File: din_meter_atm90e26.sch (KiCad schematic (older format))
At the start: 45 parts, among them J1 PCIx1, J2 Conn_01x05, J5 CONN_01X10, M1 ATM90E26_ATM90E26, M2 ATM90E26_ATM90E26, Y1 Crystal_Small, Y2 Crystal_Small

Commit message: Submitted to OSH Park & made Octopart BoM for v. A
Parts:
- J1, J2, TP_I1N_0, TP_I1N_1, TP_I1P_0, TP_I1P_1, TP_VN_0, TP_VN_1, TP_VP_0, TP_VP_1: PN (none) -> X
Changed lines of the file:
@@
 F 2 "Connectors:PCI-EXPRESS" H 8550 450 50  0001 C CNN
 F 3 "" H 8550 450 50  0001 C CNN
+F 4 "X" H 8550 1500 50  0001 C CNN "PN"
 	1    8550 1500
 	0    -1   -1   0
@@
 F 2 "MeasurementPoints:Measurement_Point_Round-SMD-Pad_Small" H 8800 1150 50  0001 C CNN
 F 3 "" H 8800 1150 50  0001 C CNN
+F 4 "X" H 8600 1150 50  0001 C CNN "PN"
 	1    8600 1150
 	0    -1   -1   0
@@
 F 2 "MeasurementPoints:Measurement_Point_Round-SMD-Pad_Small" H 7800 1150 50  0001 C CNN
 F 3 "" H 7800 1150 50  0001 C CNN
+F 4 "X" H 7600 1150 50  0001 C CNN "PN"
 	1    7600 1150
 	0    -1   -1   0
@@
 F 2 "MeasurementPoints:Measurement_Point_Round-SMD-Pad_Small" H 4150 5750 50  0001 C CNN
 F 3 "" H 4150 5750 50  0001 C CNN
+F 4 "X" H 3950 5750 50  0001 C CNN "PN"
 	1    3950 5750
 	-1   0    0    1
@@
 F 2 "MeasurementPoints:Measurement_Point_Round-SMD-Pad_Small" H 8600 5700 50  0001 C CNN
 F 3 "" H 8600 5700 50  0001 C CNN
+F 4 "X" H 8400 5700 50  0001 C CNN "PN"
 	1    8400 5700
 	-1   0    0    1
@@
 F 2 "MeasurementPoints:Measurement_Point_Round-SMD-Pad_Small" H 5300 1250 50  0001 C CNN
 F 3 "" H 5300 1250 50  0001 C CNN
+F 4 "X" H 5100 1250 50  0001 C CNN "PN"
 	1    5100 1250
 	0    -1   -1   0
@@
 F 2 "MeasurementPoints:Measurement_Point_Round-SMD-Pad_Small" H 5950 1200 50  0001 C CNN
 F 3 "" H 5950 1200 50  0001 C CNN
+F 4 "X" H 5750 1200 50  0001 C CNN "PN"
 	1    5750 1200
 	0    -1   -1   0
@@
 F 2 "MeasurementPoints:Measurement_Point_Round-SMD-Pad_Small" H 6450 1250 50  0001 C CNN
 F 3 "" H 6450 1250 50  0001 C CNN
+F 4 "X" H 6250 1250 50  0001 C CNN "PN"
 	1    6250 1250
 	0    -1   -1   0
@@
 F 2 "MeasurementPoints:Measurement_Point_Round-SMD-Pad_Small" H 7000 1250 50  0001 C CNN
 F 3 "" H 7000 1250 50  0001 C CNN
+F 4 "X" H 6800 1250 50  0001 C CNN "PN"
 	1    6800 1250
 	0    -1   -1   0
@@
 F 2 "FitHome_conn:conn_5_2.54mm" H 10250 2250 50  0001 C CNN
 F 3 "~" H 10250 2250 50  0001 C CNN
+F 4 "X" H 10250 2250 50  0001 C CNN "PN"
 	1    10250 2250
 	0    -1   -1   0

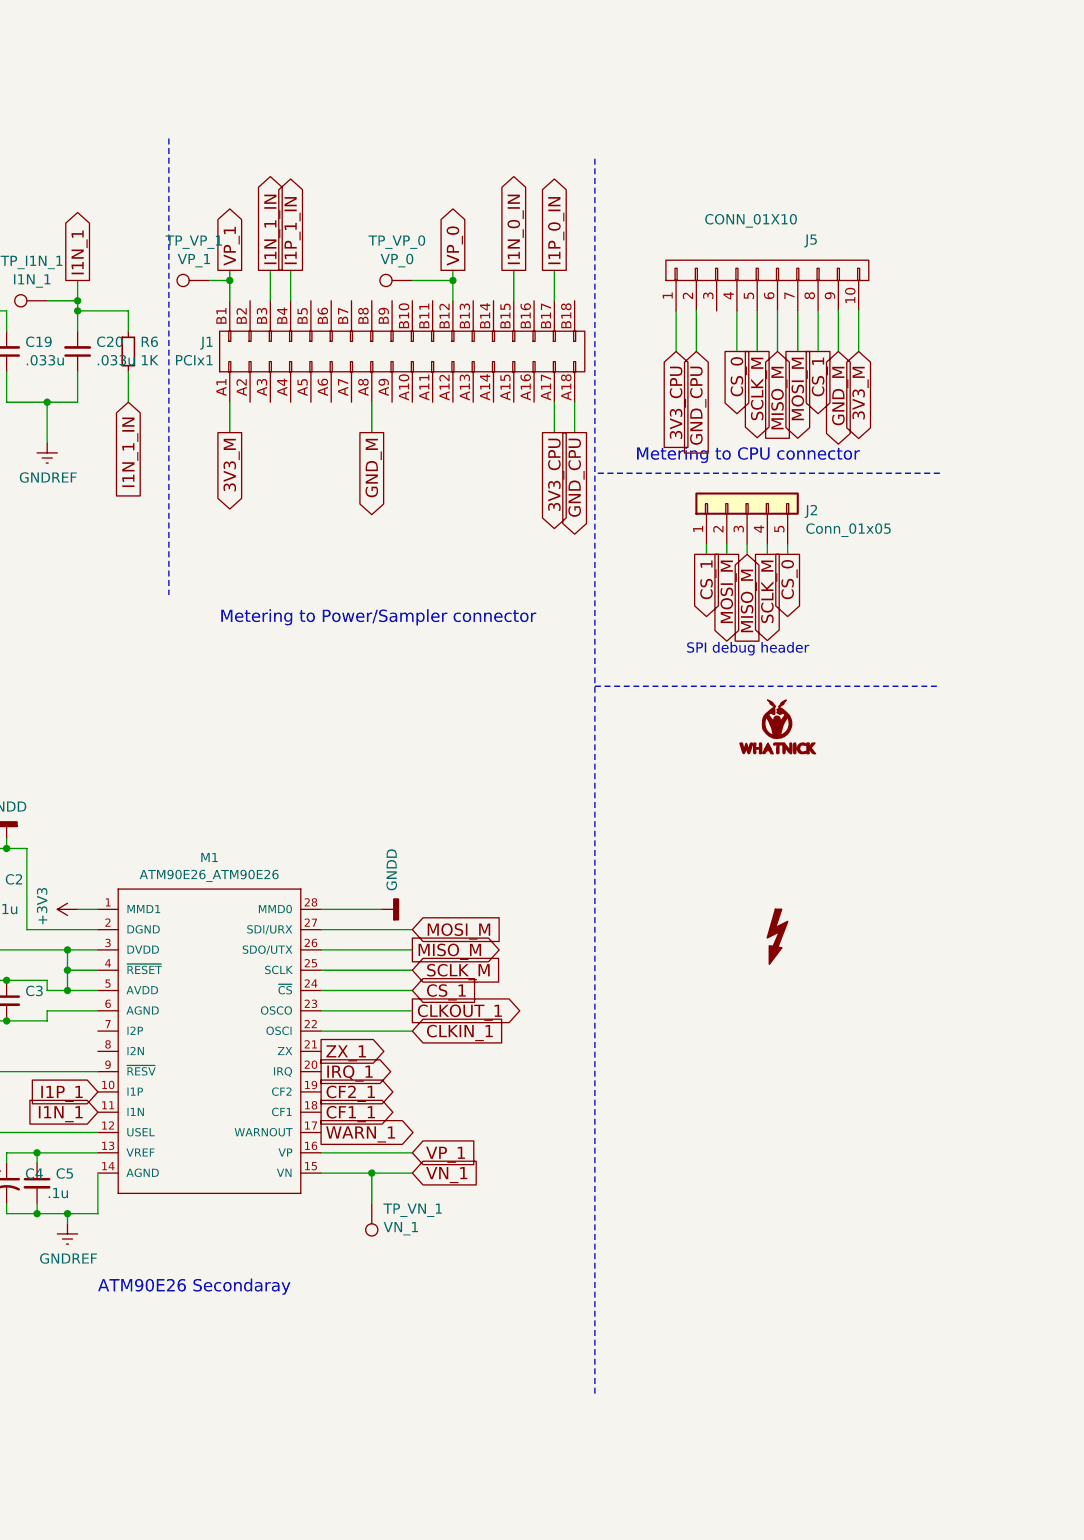
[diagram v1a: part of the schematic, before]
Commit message: updated readme.
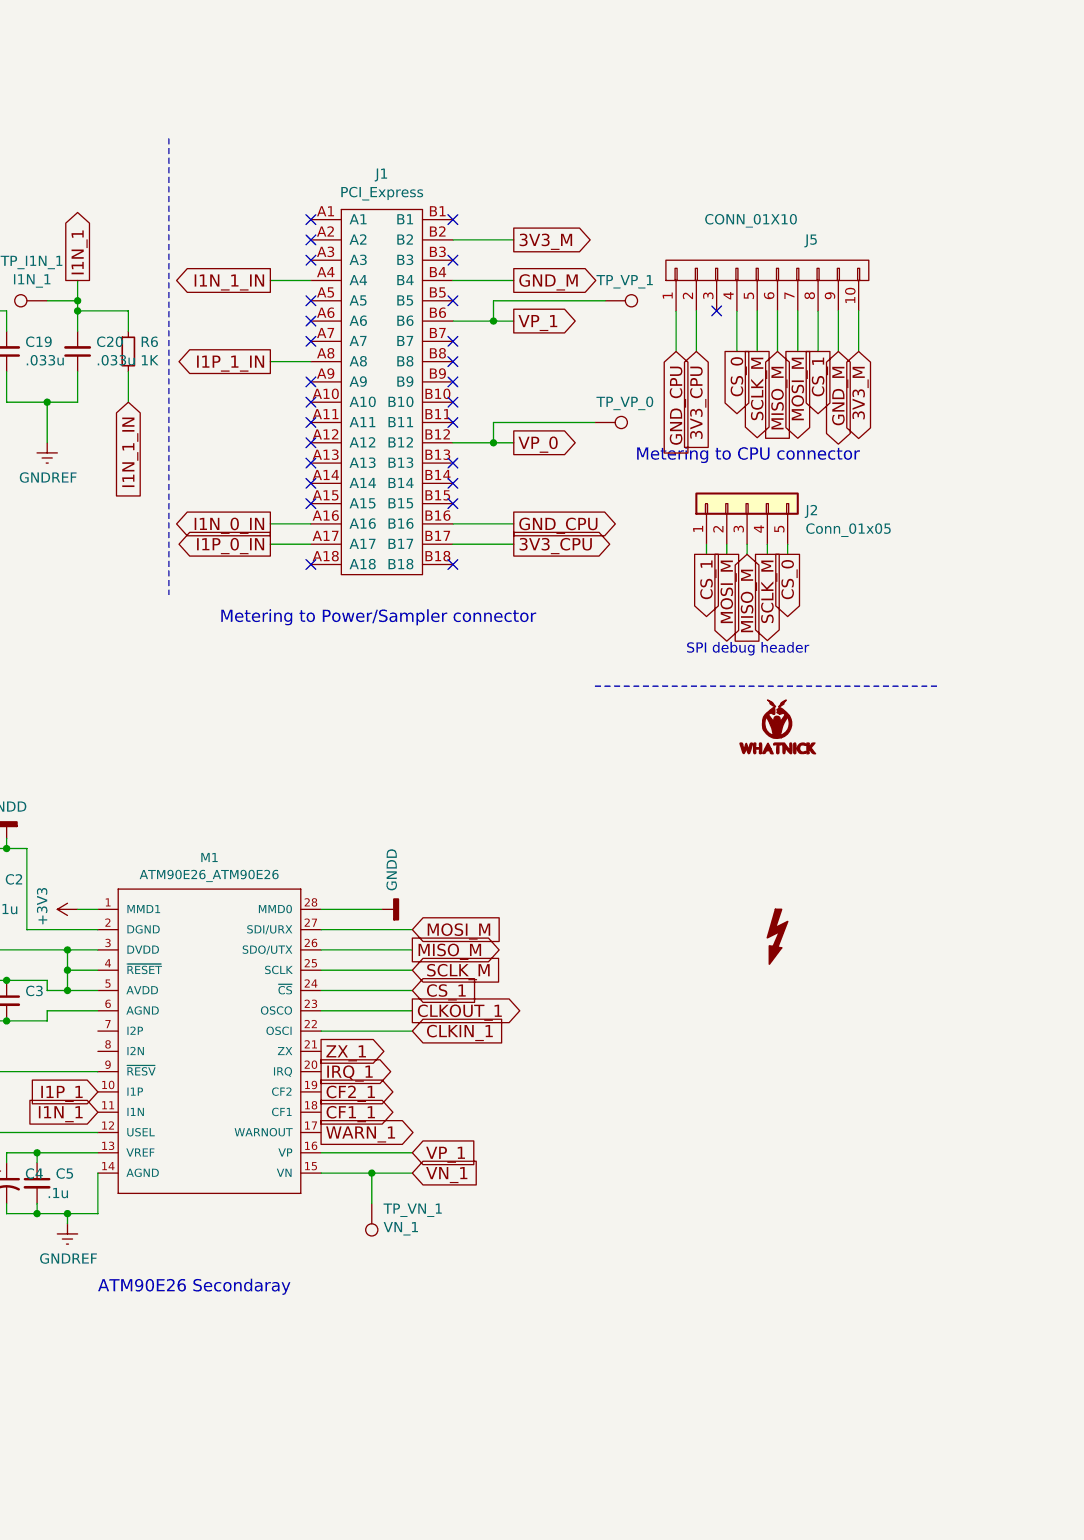
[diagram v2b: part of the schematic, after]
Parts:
- removed J1: PCIx1, Connectors:PCI-EXPRESS, symbol din_meter_atm90e26-rescue:PCIx1
- added J1: PCI_Express, FitHome_conn:PCI-EXPRESS, symbol FitHome:PCI_Express
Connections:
- net 3V3_CPU: now also J5.2 (P2), J1.B17; no longer J5.1 (P1)
- net 3V3_M: now also J1.B2
- net GND_CPU: now also J5.1 (P1), J1.B16; no longer J5.2 (P2)
- net GND_M: now also J1.B4
- net I1N_0_IN: now also J1.A16
- net I1N_1_IN: now also J1.A4
- net I1P_0_IN: now also J1.A17
- net I1P_1_IN: now also J1.A8
- net VP_0: now also J1.B12
- net VP_1: now also J1.B6
- no-connect marks 0 -> 27
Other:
- moved on the sheet: TP_VP_0, TP_VP_1
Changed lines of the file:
@@
 Text GLabel 10800 1500 3    60   BiDi ~ 0
 3V3_M
+Text GLabel 10000 1500 3    60   Input ~ 0
+3V3_CPU
 Text GLabel 9900 1500 3    60   Input ~ 0
-3V3_CPU
-Text GLabel 10000 1500 3    60   Input ~ 0
 GND_CPU
 Text GLabel 10500 1500 3    60   Output ~ 0
@@
 	1    0    0    -1
 $EndComp
-Text GLabel 7700 1900 3    60   Output ~ 0
+Text GLabel 9100 950  2    60   Output ~ 0
 3V3_M
-Text GLabel 8800 1100 1    60   Output ~ 0
+Text GLabel 9100 1950 2    60   Output ~ 0
 VP_0
-Text GLabel 7700 1100 1    60   Output ~ 0
+Text GLabel 9100 1350 2    60   Output ~ 0
 VP_1
-Text GLabel 8400 1900 3    60   Output ~ 0
+Text GLabel 9100 1150 2    60   Output ~ 0
 GND_M
-Text GLabel 9300 1900 3    60   Output ~ 0
+Text GLabel 9100 2450 2    60   Output ~ 0
 3V3_CPU
-Text GLabel 9400 1900 3    60   Output ~ 0
+Text GLabel 9100 2350 2    60   Output ~ 0
 GND_CPU
-Text GLabel 9300 1100 1    60   Output ~ 0
+Text GLabel 7900 2450 0    60   Output ~ 0
 I1P_0_IN
-Text GLabel 9100 1100 1    60   Output ~ 0
+Text GLabel 7900 2350 0    60   Output ~ 0
 I1N_0_IN
-Text GLabel 8000 1100 1    60   Output ~ 0
+Text GLabel 7900 1550 0    60   Output ~ 0
 I1P_1_IN
-Text GLabel 7900 1100 1    60   Output ~ 0
+Text GLabel 7900 1150 0    60   Output ~ 0
 I1N_1_IN
 $Comp
@@
 	10200 1300 10200 1500
 Wire Wire Line
-	10000 1300 10000 1500
-Wire Wire Line
 	9900 1300 9900 1500
 Connection ~ 6600 4800
@@
 	6900 4650 7050 4650
 Wire Wire Line
-	7900 1100 7900 1250
-Wire Wire Line
-	8000 1100 8000 1250
-Wire Wire Line
-	9100 1100 9100 1250
-Wire Wire Line
-	9300 1100 9300 1250
-Wire Wire Line
 	1350 5050 1850 5050
 Wire Notes Line
@@
 Wire Wire Line
 	2200 4350 2600 4350
-Wire Wire Line
-	8400 1750 8400 1900
-Wire Wire Line
-	7700 1750 7700 1900
-$Comp
-L din_meter_atm90e26-rescue:PCIx1 J1
-U 1 1 5C98D347
-P 8550 1500
-F 0 "J1" V 8596 2428 50  0000 L CNN
-F 1 "PCIx1" V 8505 2428 50  0000 L CNN
-F 2 "Connectors:PCI-EXPRESS" H 8550 450 50  0001 C CNN
-F 3 "" H 8550 450 50  0001 C CNN
-F 4 "X" H 8550 1500 50  0001 C CNN "PN"
-	1    8550 1500
-	0    -1   -1   0
-$EndComp
-Wire Wire Line
-	7700 1250 7700 1150
-Wire Wire Line
-	9300 1900 9300 1750
-Wire Wire Line
-	9400 1900 9400 1750
-Wire Wire Line
-	8800 1100 8800 1150
 $Comp
 L conn:TEST_1P TP_VP_0
 U 1 1 5C98E37F
-P 8600 1150
-F 0 "TP_VP_0" V 8795 1224 50  0000 C CNN
-F 1 "VP_0" V 8704 1224 50  0000 C CNN
-F 2 "MeasurementPoints:Measurement_Point_Round-SMD-Pad_Small" H 8800 1150 50  0001 C CNN
-F 3 "" H 8800 1150 50  0001 C CNN
-F 4 "X" H 8600 1150 50  0001 C CNN "PN"
-	1    8600 1150
-	0    -1   -1   0
-$EndComp
-Wire Wire Line
-	8600 1150 8800 1150
-Connection ~ 8800 1150
-Wire Wire Line
-	8800 1150 8800 1250
+P 9500 1850
+F 0 "TP_VP_0" V 9400 2000 50  0000 C CNN
+F 1 "VP_0" V 9604 1924 50  0001 C CNN
+F 2 "MeasurementPoints:Measurement_Point_Round-SMD-Pad_Small" H 9700 1850 50  0001 C CNN
+F 3 "" H 9700 1850 50  0001 C CNN
+F 4 "X" H 9500 1850 50  0001 C CNN "PN"
+	1    9500 1850
+	0    1    1    0
+$EndComp
 $Comp
 L conn:TEST_1P TP_VP_1
 U 1 1 5C999048
-P 7600 1150
-F 0 "TP_VP_1" V 7795 1224 50  0000 C CNN
-F 1 "VP_1" V 7704 1224 50  0000 C CNN
-F 2 "MeasurementPoints:Measurement_Point_Round-SMD-Pad_Small" H 7800 1150 50  0001 C CNN
-F 3 "" H 7800 1150 50  0001 C CNN
-F 4 "X" H 7600 1150 50  0001 C CNN "PN"
-	1    7600 1150
-	0    -1   -1   0
-$EndComp
-Wire Wire Line
-	7600 1150 7700 1150
-Connection ~ 7700 1150
-Wire Wire Line
-	7700 1150 7700 1100
+P 9550 1250
+F 0 "TP_VP_1" V 9450 1350 50  0000 C CNN
+F 1 "VP_1" V 9654 1324 50  0001 C CNN
+F 2 "MeasurementPoints:Measurement_Point_Round-SMD-Pad_Small" H 9750 1250 50  0001 C CNN
+F 3 "" H 9750 1250 50  0001 C CNN
+F 4 "X" H 9550 1250 50  0001 C CNN "PN"
+	1    9550 1250
+	0    1    1    0
+$EndComp
 $Comp
 L conn:TEST_1P TP_VN_0
@@
 Text Notes 9950 3000 0    50   ~ 0
 SPI debug header
-Wire Notes Line
-	11200 2100 9500 2100
-Wire Notes Line
-	9500 550  9500 6650
 Text GLabel 10050 2500 3    60   Output ~ 0
 CS_1
@@
 Wire Notes Line
 	9500 3150 11200 3150
+$Comp
+L FitHome:PCI_Express J1
+U 1 1 5CA91AA9
+P 8350 2350
+F 0 "J1" H 8450 4075 50  0000 C CNN
+F 1 "PCI_Express" H 8450 3984 50  0000 C CNN
+F 2 "FitHome_conn:PCI-EXPRESS" H 8350 2350 50  0001 C CNN
+F 3 "" H 8350 2350 50  0001 C CNN
+	1    8350 2350
+	1    0    0    -1
+$EndComp
+Wire Wire Line
+	8800 950  9100 950
+Wire Wire Line
+	9100 1150 8800 1150
+NoConn ~ 8800 850
+NoConn ~ 8800 1050
+NoConn ~ 8800 1250
+Wire Wire Line
+	9100 1350 9000 1350
+Wire Wire Line
+	9550 1250 9000 1250
+Wire Wire Line
+	9000 1250 9000 1350
+Connection ~ 9000 1350
+Wire Wire Line
+	9000 1350 8800 1350
+Wire Wire Line
+	9100 1950 9000 1950
+Wire Wire Line
+	9500 1850 9000 1850
+Wire Wire Line
+	9000 1850 9000 1950
+Connection ~ 9000 1950
+Wire Wire Line
+	9000 1950 8800 1950
+Wire Wire Line
+	7900 2450 8100 2450
+Wire Wire Line
+	9100 2450 8800 2450
+NoConn ~ 8800 2550
+Wire Wire Line
+	10000 1300 10000 1500
+Wire Wire Line
+	9100 2350 8800 2350
+NoConn ~ 8800 1450
+NoConn ~ 8800 1550
+NoConn ~ 8800 1650
+NoConn ~ 8800 1750
+NoConn ~ 8800 1850
+NoConn ~ 8800 2050
+NoConn ~ 8800 2150
+NoConn ~ 8800 2250
+NoConn ~ 10100 1300
+Wire Wire Line
+	8100 2350 7900 2350
+Wire Wire Line
+	7900 1550 8100 1550
+Wire Wire Line
+	8100 1150 7900 1150
+NoConn ~ 8100 2550
+NoConn ~ 8100 2250
+NoConn ~ 8100 2150
+NoConn ~ 8100 2050
+NoConn ~ 8100 1950
+NoConn ~ 8100 1850
+NoConn ~ 8100 1750
+NoConn ~ 8100 1650
+NoConn ~ 8100 1450
+NoConn ~ 8100 1350
+NoConn ~ 8100 1250
+NoConn ~ 8100 1050
+NoConn ~ 8100 950
+NoConn ~ 8100 850
 $EndSCHEMATC

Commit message: OSH Park Rev B
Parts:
- J1: symbol FitHome:PCI_Express -> din_meter_atm90e26-rescue:PCI_Express-FitHome
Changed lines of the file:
@@
 	9500 3150 11200 3150
 $Comp
-L FitHome:PCI_Express J1
+L din_meter_atm90e26-rescue:PCI_Express-FitHome J1
 U 1 1 5CA91AA9
 P 8350 2350
